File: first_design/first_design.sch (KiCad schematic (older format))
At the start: 44 parts, among them IC1 BD48K60, IC2 AZ2085, IC3 AP65450, IC4 RN, IC5 VNH7070BAS, J1 Conn_02x20_Odd_Even, J2 Accelerometer_small, J3 Accelerometer_standard, J4 Servo_motor

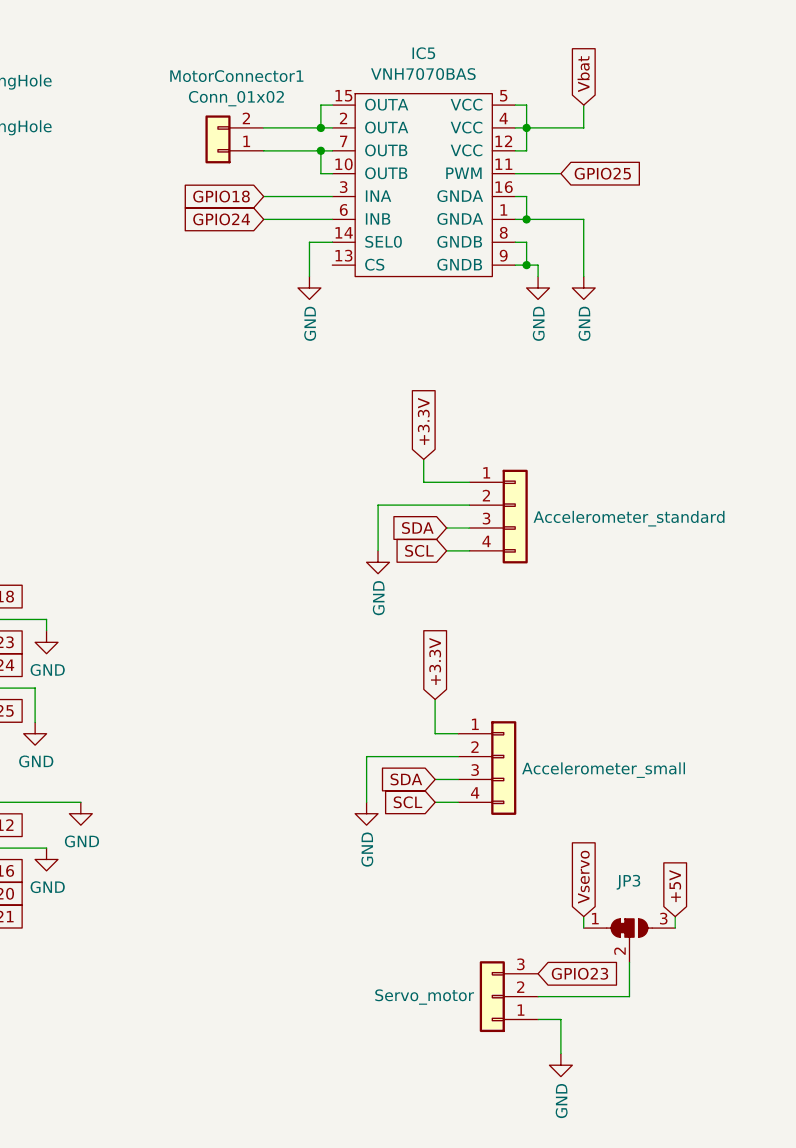
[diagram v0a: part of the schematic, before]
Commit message: Killing it
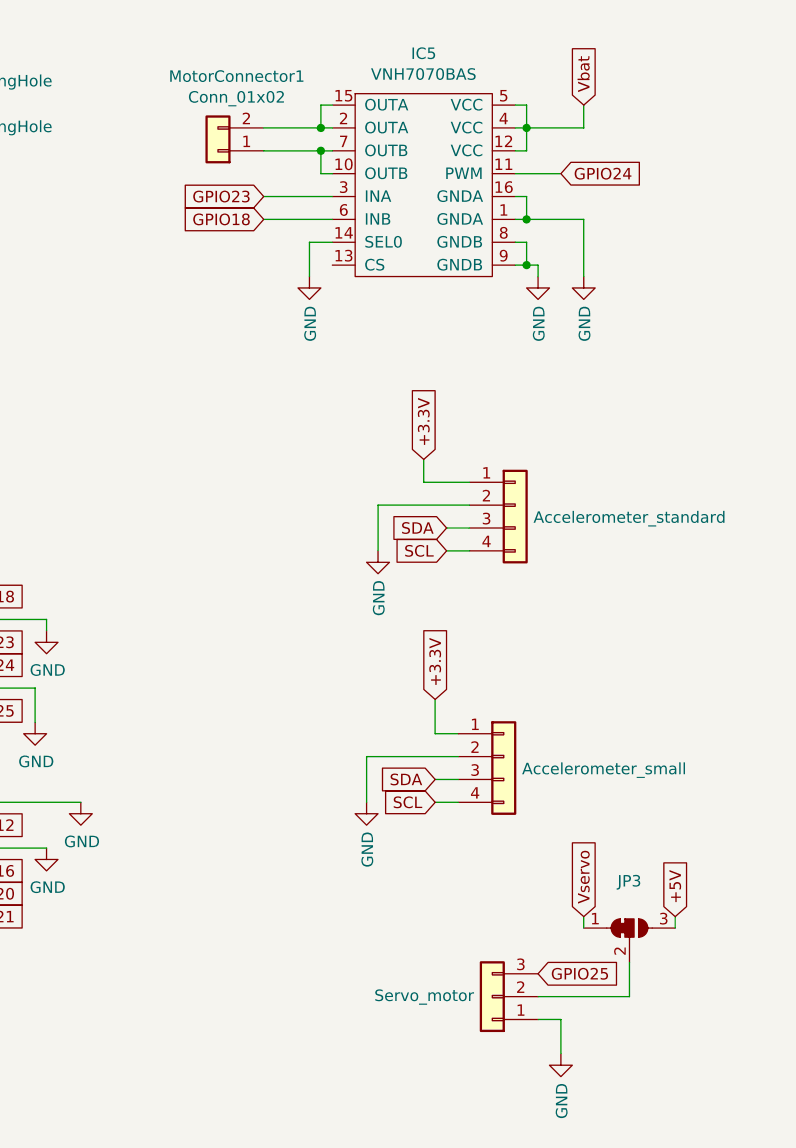
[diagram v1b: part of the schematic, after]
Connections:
- net GPIO18: now also IC5.6 (INB); no longer IC5.3 (INA)
- net GPIO23: now also IC5.3 (INA); no longer J4.3 (Pin_3)
- net GPIO24: now also IC5.11 (PWM); no longer IC5.6 (INB)
- net GPIO25: now also J4.3 (Pin_3); no longer IC5.11 (PWM)
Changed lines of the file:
@@
 	8950 1050 9200 1050
 Connection ~ 9200 1050
-Text GLabel 8950 1250 0    50   Input ~ 0
+Text GLabel 8950 1350 0    50   Input ~ 0
 GPIO18
-Text GLabel 8950 1350 0    50   Input ~ 0
+Text GLabel 10250 1150 2    50   Input ~ 0
 GPIO24
 Wire Wire Line
-	8950 1250 9250 1250
+	8950 1350 9250 1350
 Text GLabel 7550 3000 2    50   Input ~ 0
 GPIO18
@@
 	1    0    0    -1
 $EndComp
-Text GLabel 10150 4650 2    50   Input ~ 0
+Text GLabel 8950 1250 0    50   Input ~ 0
 GPIO23
 Wire Wire Line
@@
 	9150 1450 9150 1600
 Wire Wire Line
-	9250 1350 8950 1350
+	9250 1250 8950 1250
 $Comp
 L first_design-rescue:RN-Connector IC4
@@
 Wire Wire Line
 	7000 2500 7000 2400
-Text GLabel 10250 1150 2    50   Input ~ 0
+Text GLabel 10150 4650 2    50   Input ~ 0
 GPIO25
 Text GLabel 7550 3200 2    50   Input ~ 0
